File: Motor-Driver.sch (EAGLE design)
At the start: 7 parts, among them M1 MOTOR_PADS, Q1 CJ2302

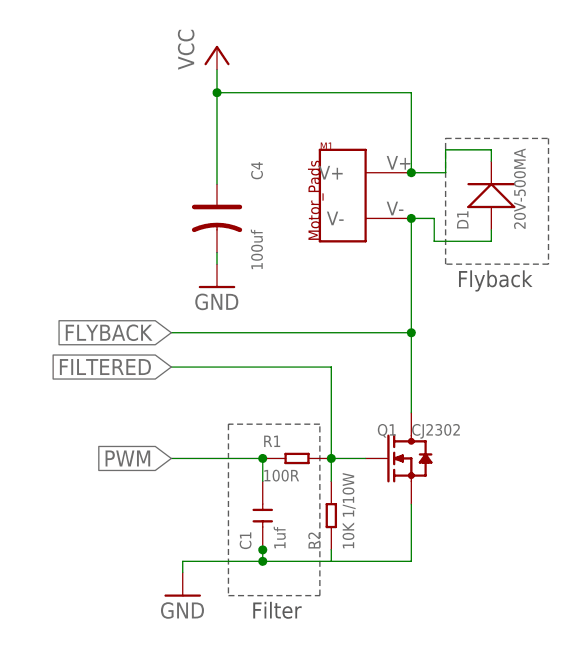
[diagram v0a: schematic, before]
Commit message: fix filter
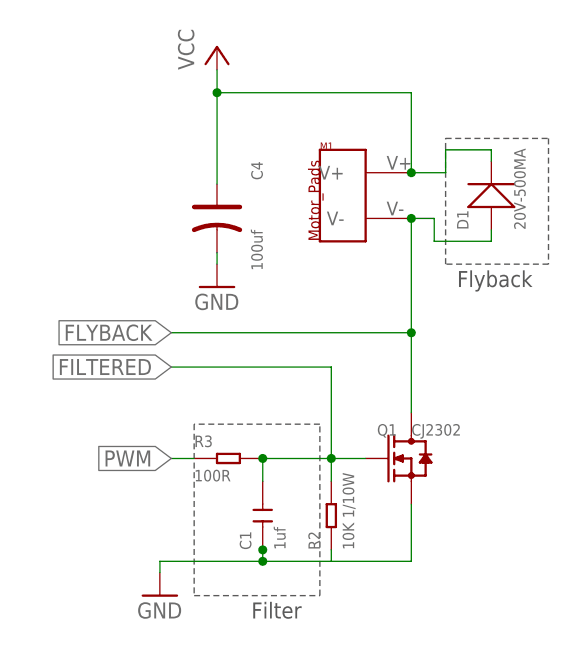
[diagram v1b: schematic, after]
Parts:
- removed R1: 100R, Seeed-Resistor-2016:SMD-RES-100R-5%-1/10W(0603)
- added R3: 100R, Seeed-Resistor-2016:SMD-RES-100R-5%-1/10W(0603)
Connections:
- net FILTERED: now also C1.2, R3.2; no longer R1.2
- net PWM: now also R3.1; no longer C1.2, R1.1
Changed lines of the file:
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@@
 <setting verticaltext="up"/>
 </settings>
-<grid distance="0.1" unitdist="inch" unit="inch" style="lines" multiple="1" display="no" altdistance="0.01" altunitdist="inch" altunit="inch"/>
+<grid distance="0.05" unitdist="inch" unit="inch" style="lines" multiple="1" display="no" altdistance="0.01" altunitdist="inch" altunit="inch"/>
 <layers>
 <layer number="1" name="Top" color="4" fill="1" visible="no" active="no"/>
@@
 <parts>
 <part name="Q1" library="Seeed-Transistor-2016" deviceset="SMD-MOSFET-N-CH-20V-2.1A-CJ2302(SOT-23)" device="" value="CJ2302"/>
-<part name="R1" library="Seeed-Resistor-2016" deviceset="SMD-RES-100R-5%-1/10W(0603)" device="" value="100R"/>
 <part name="R2" library="Seeed-Resistor-2016" deviceset="SMD-RES-10K-5%-1/10W(0603)" device="" value="10K 1/10W"/>
 <part name="C1" library="Seeed-Capacitor-2016" deviceset="CERAMIC-1UF-10V-10%-X5R(0402)" device="" value="1uf"/>
@@
 <part name="D1" library="Seeed-Diode-2016" deviceset="SMD-DIODE-SCHOTTKY-20V-500MA(SOD-123)" device="" value="20V-500MA"/>
 <part name="FRAME1" library="frames" deviceset="FRAME_A_L" device=""/>
+<part name="R3" library="Seeed-Resistor-2016" deviceset="SMD-RES-100R-5%-1/10W(0603)" device="" value="100R"/>
 </parts>
 <sheets>
 <sheet>
 <plain>
-<wire x1="127" y1="102.87" x2="127" y2="83.82" width="0.1524" layer="97" style="shortdash"/>
-<wire x1="127" y1="83.82" x2="137.16" y2="83.82" width="0.1524" layer="97" style="shortdash"/>
+<wire x1="123.19" y1="102.87" x2="123.19" y2="83.82" width="0.1524" layer="97" style="shortdash"/>
+<wire x1="123.19" y1="83.82" x2="137.16" y2="83.82" width="0.1524" layer="97" style="shortdash"/>
 <wire x1="137.16" y1="83.82" x2="137.16" y2="102.87" width="0.1524" layer="97" style="shortdash"/>
-<wire x1="137.16" y1="102.87" x2="127" y2="102.87" width="0.1524" layer="97" style="shortdash"/>
+<wire x1="137.16" y1="102.87" x2="123.19" y2="102.87" width="0.1524" layer="97" style="shortdash"/>
 <text x="129.54" y="81.28" size="1.778" layer="97">Filter</text>
 <wire x1="151.13" y1="134.62" x2="162.56" y2="134.62" width="0.1524" layer="97" style="shortdash"/>
@@
 <instances>
 <instance part="Q1" gate="G$1" x="147.32" y="99.06"/>
-<instance part="R1" gate="G$1" x="134.62" y="99.06"/>
 <instance part="R2" gate="G$1" x="138.43" y="92.71" rot="R90"/>
 <instance part="C1" gate="G$1" x="130.81" y="92.71" rot="R90"/>
 <instance part="C4" gate="G$1" x="125.73" y="125.73" rot="R270"/>
-<instance part="GND1" gate="1" x="121.92" y="83.82"/>
+<instance part="GND1" gate="1" x="119.38" y="83.82"/>
 <instance part="GND2" gate="1" x="125.73" y="118.11"/>
 <instance part="P+1" gate="VCC" x="125.73" y="144.78"/>
@@
 <instance part="FRAME1" gate="G$1" x="0" y="0"/>
 <instance part="FRAME1" gate="G$2" x="172.72" y="0"/>
+<instance part="R3" gate="G$1" x="127" y="99.06"/>
 </instances>
 <busses>
@@
 <junction x="130.81" y="87.63"/>
 <pinref part="GND1" gate="1" pin="GND"/>
-<wire x1="121.92" y1="86.36" x2="121.92" y2="87.63" width="0.1524" layer="91"/>
-<wire x1="121.92" y1="87.63" x2="130.81" y2="87.63" width="0.1524" layer="91"/>
+<wire x1="119.38" y1="86.36" x2="119.38" y2="87.63" width="0.1524" layer="91"/>
+<wire x1="119.38" y1="87.63" x2="130.81" y2="87.63" width="0.1524" layer="91"/>
 <wire x1="130.81" y1="87.63" x2="138.43" y2="87.63" width="0.1524" layer="91"/>
 <wire x1="138.43" y1="88.9" x2="138.43" y2="87.63" width="0.1524" layer="91"/>
@@
 <net name="PWM" class="0">
 <segment>
-<pinref part="R1" gate="G$1" pin="1"/>
-<wire x1="130.81" y1="96.52" x2="130.81" y2="99.06" width="0.1524" layer="91"/>
-<junction x="130.81" y="99.06"/>
-<pinref part="C1" gate="G$1" pin="2"/>
-<wire x1="120.65" y1="99.06" x2="130.81" y2="99.06" width="0.1524" layer="91"/>
+<pinref part="R3" gate="G$1" pin="1"/>
+<wire x1="120.65" y1="99.06" x2="123.19" y2="99.06" width="0.1524" layer="91"/>
 <label x="120.65" y="99.06" size="1.778" layer="95" rot="R180" xref="yes"/>
-</segment>
-</net>
-<net name="FILTERED" class="0">
-<segment>
-<pinref part="R1" gate="G$1" pin="2"/>
-<pinref part="R2" gate="G$1" pin="2"/>
-<wire x1="138.43" y1="99.06" x2="138.43" y2="96.52" width="0.1524" layer="91"/>
-<pinref part="Q1" gate="G$1" pin="G"/>
-<junction x="138.43" y="99.06"/>
-<wire x1="138.43" y1="99.06" x2="142.24" y2="99.06" width="0.1524" layer="91"/>
-<wire x1="138.43" y1="99.06" x2="138.43" y2="109.22" width="0.1524" layer="91"/>
-<wire x1="138.43" y1="109.22" x2="120.65" y2="109.22" width="0.1524" layer="91"/>
-<label x="120.65" y="109.22" size="1.778" layer="95" rot="R180" xref="yes"/>
 </segment>
 </net>
@@
 </segment>
 </net>
+<net name="FILTERED" class="0">
+<segment>
+<wire x1="130.81" y1="96.52" x2="130.81" y2="99.06" width="0.1524" layer="91"/>
+<junction x="130.81" y="99.06"/>
+<pinref part="C1" gate="G$1" pin="2"/>
+<pinref part="R3" gate="G$1" pin="2"/>
+<pinref part="R2" gate="G$1" pin="2"/>
+<wire x1="138.43" y1="99.06" x2="138.43" y2="96.52" width="0.1524" layer="91"/>
+<pinref part="Q1" gate="G$1" pin="G"/>
+<junction x="138.43" y="99.06"/>
+<wire x1="138.43" y1="99.06" x2="142.24" y2="99.06" width="0.1524" layer="91"/>
+<wire x1="138.43" y1="99.06" x2="138.43" y2="109.22" width="0.1524" layer="91"/>
+<wire x1="138.43" y1="109.22" x2="120.65" y2="109.22" width="0.1524" layer="91"/>
+<label x="120.65" y="109.22" size="1.778" layer="95" rot="R180" xref="yes"/>
+<wire x1="130.81" y1="99.06" x2="138.43" y2="99.06" width="0.1524" layer="91"/>
+</segment>
+</net>
